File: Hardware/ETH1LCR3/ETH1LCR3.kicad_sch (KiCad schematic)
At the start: 5 parts

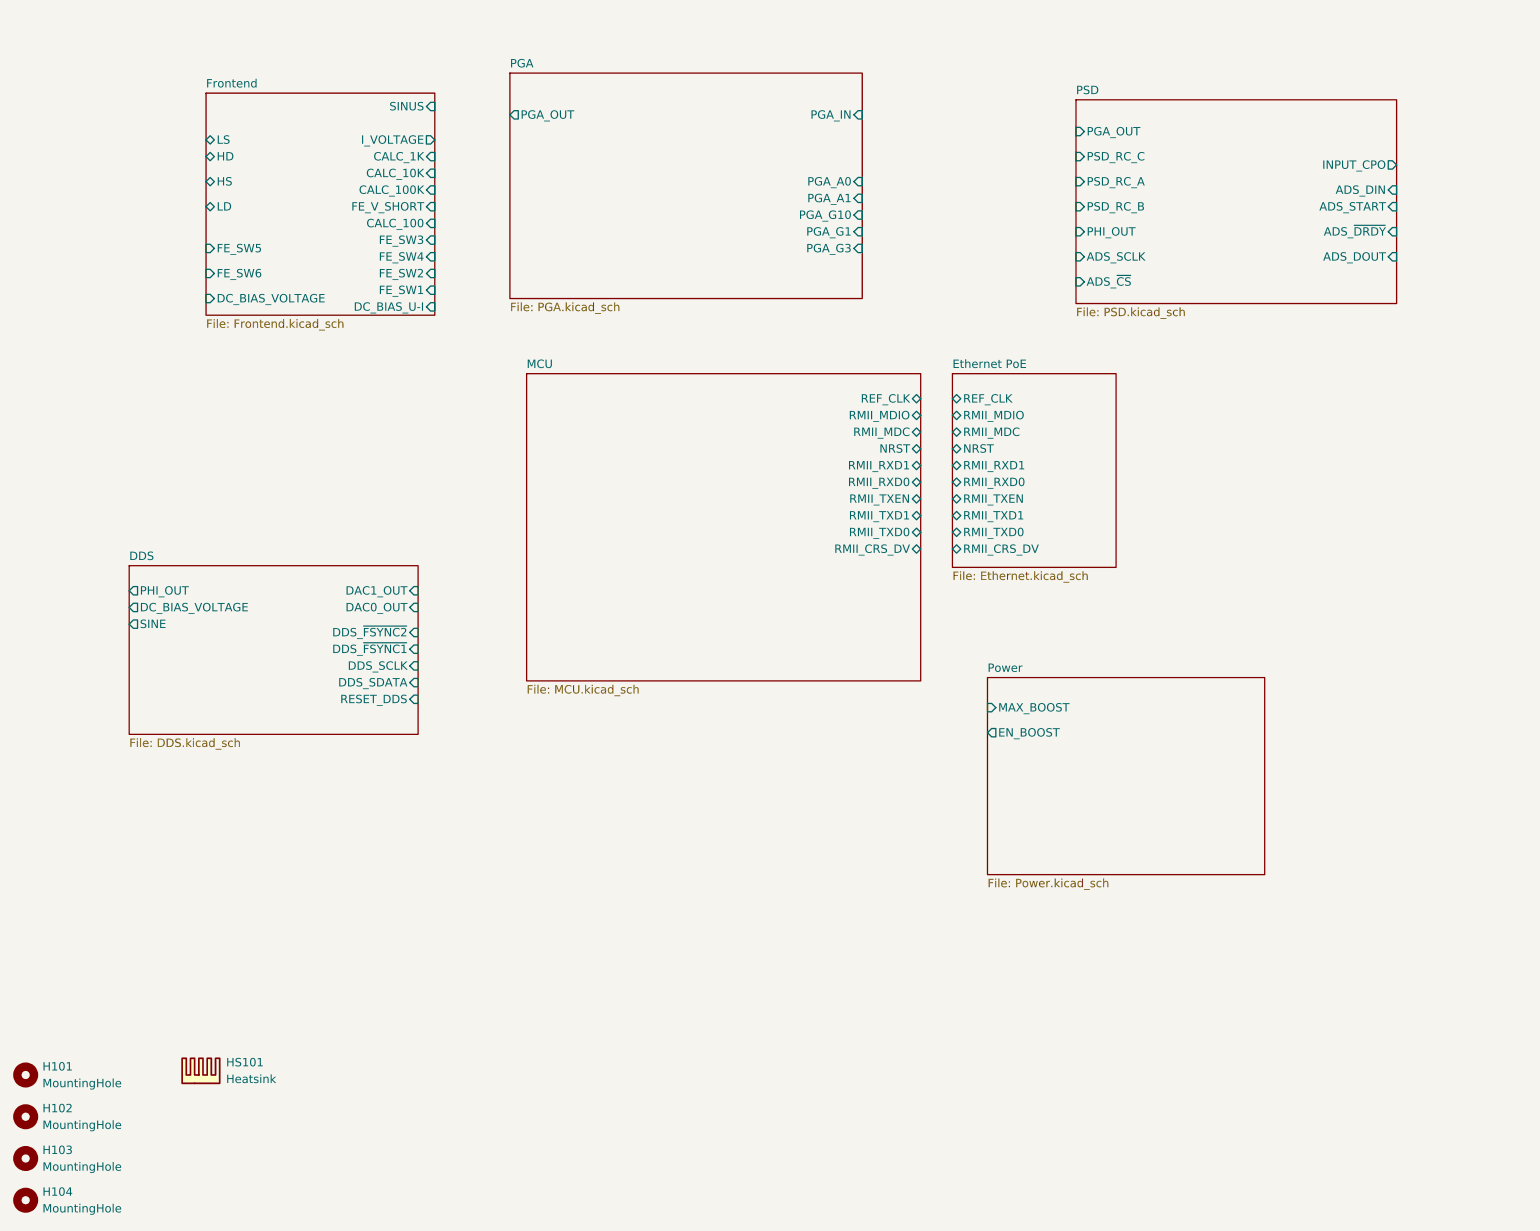
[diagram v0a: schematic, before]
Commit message: Hardware
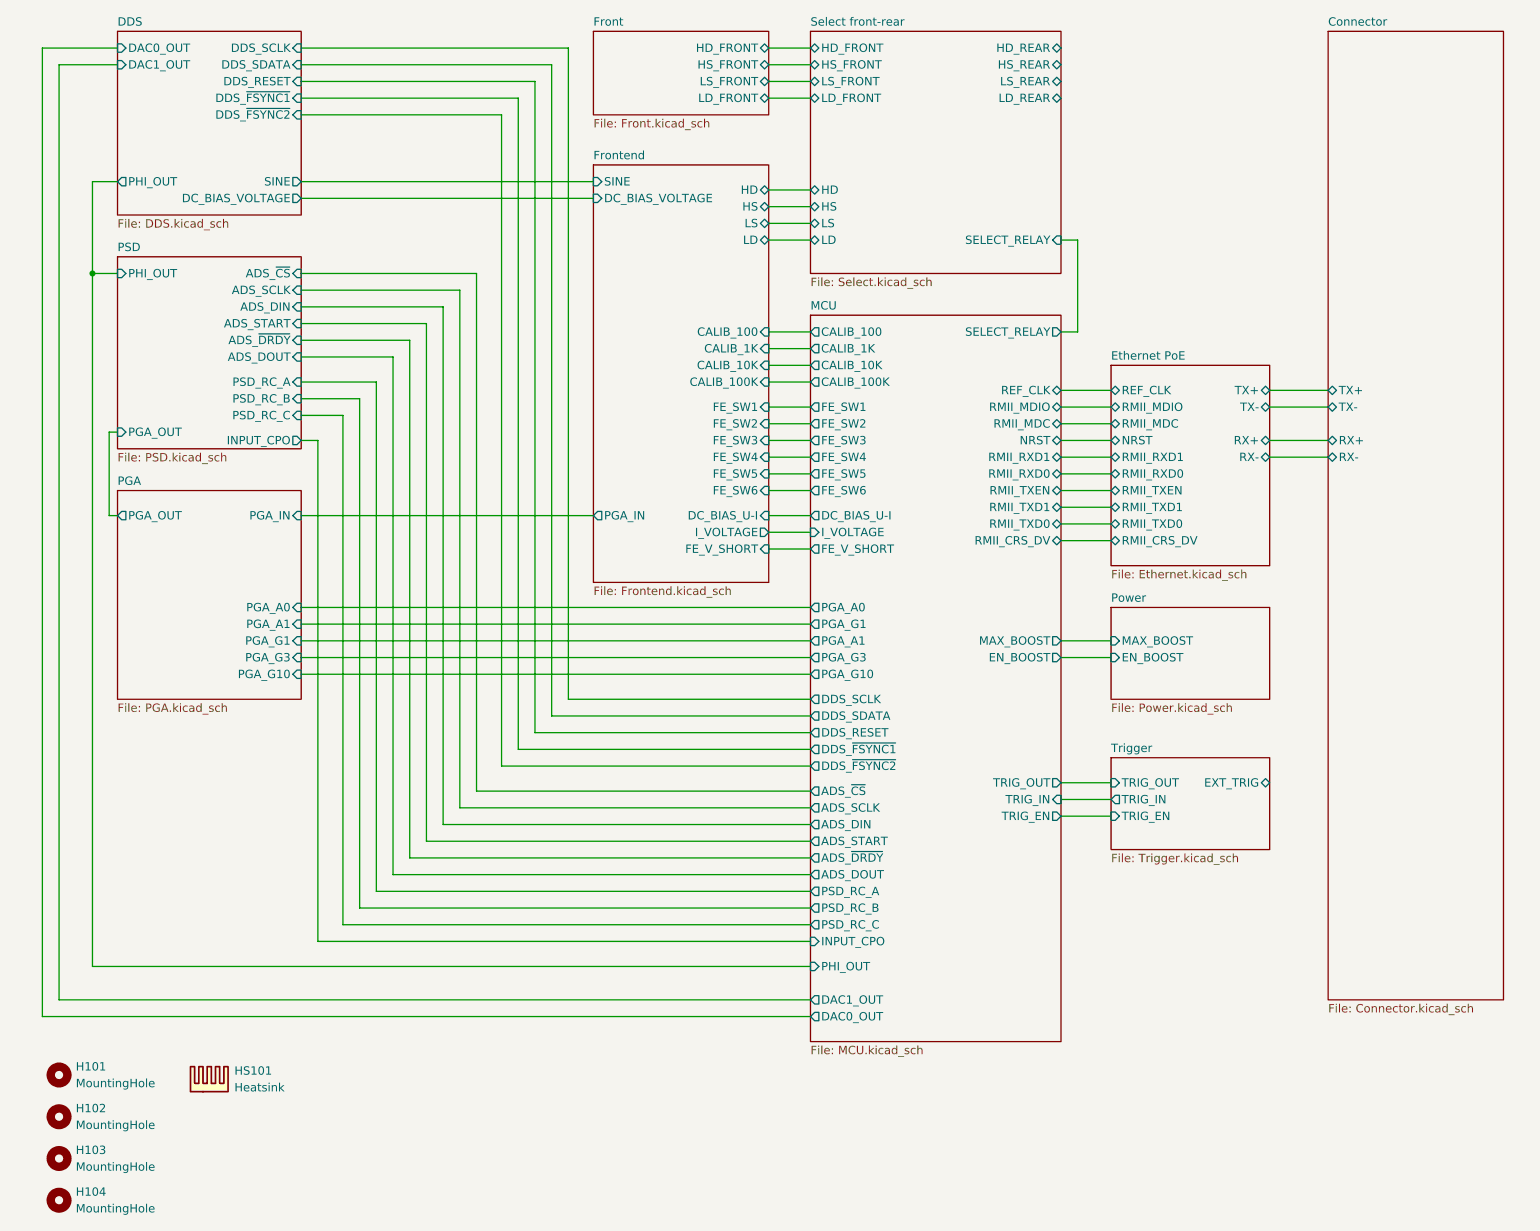
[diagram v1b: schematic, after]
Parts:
- H101, H102, H103, H104: footprint (none) -> MountingHole:MountingHole_3.2mm_M3_DIN965_Pad
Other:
- added sheet Connector (Connector.kicad_sch)
- added sheet Front (Front.kicad_sch)
- added sheet Select front-rear (Select.kicad_sch)
- added sheet Trigger (Trigger.kicad_sch)
- sheet DDS ports: added DDS_RESET; removed RESET_DDS
- sheet Ethernet PoE ports: added RX+, RX-, TX+, TX-; removed none
- sheet Frontend ports: added CALIB_100, CALIB_100K, CALIB_10K, CALIB_1K, PGA_IN, SINE; removed CALC_100, CALC_100K, CALC_10K, CALC_1K, SINUS
- sheet MCU ports: added ADS_DIN, ADS_DOUT, ADS_SCLK, ADS_START, ADS_~{CS}, ADS_~{DRDY}, CALIB_100, CALIB_100K, CALIB_10K, CALIB_1K, DAC0_OUT, DAC1_OUT, DC_BIAS_U-I, DDS_RESET, DDS_SCLK, DDS_SDATA, DDS_~{FSYNC1}, DDS_~{FSYNC2}, EN_BOOST, FE_SW1, FE_SW2, FE_SW3, FE_SW4, FE_SW5, FE_SW6, FE_V_SHORT, INPUT_CPO, I_VOLTAGE, MAX_BOOST, PGA_A0, PGA_A1, PGA_G1, PGA_G10, PGA_G3, PHI_OUT, PSD_RC_A, PSD_RC_B, PSD_RC_C, SELECT_RELAY, TRIG_EN, TRIG_IN, TRIG_OUT; removed none
- moved on the sheet: H101, H102, H103, H104, HS101
